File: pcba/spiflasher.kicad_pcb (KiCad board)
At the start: 2 copper layers, 62.5 x 25.7 mm, 41 parts, among them J1 USB_B_Micro, J2 Conn_02x04_Counter_Clockwise, J3 Conn_01x10, J4 Conn_01x10, U1 FT232H, U2 93LC56BT-I/OT, U3 TXB0104PW, Y1 12 MHz

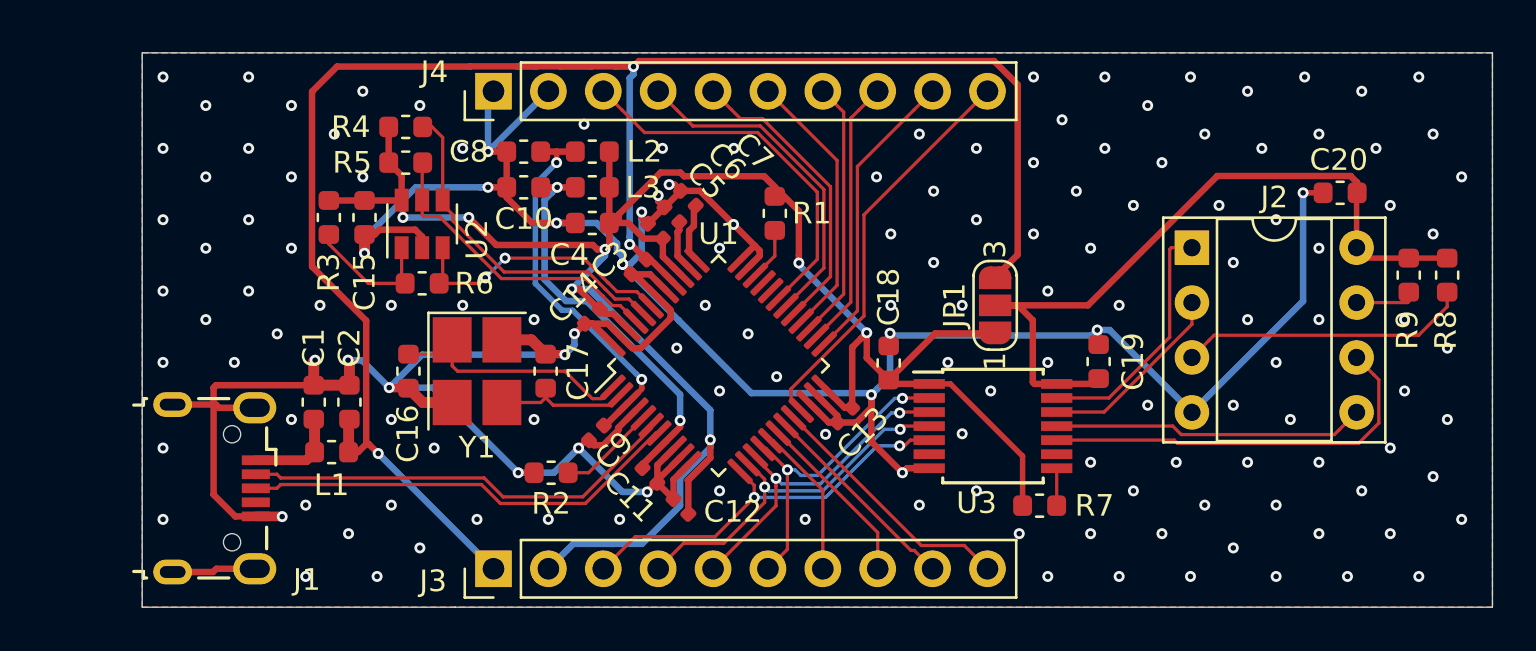
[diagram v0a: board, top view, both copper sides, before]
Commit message: Removed unnecessary components.
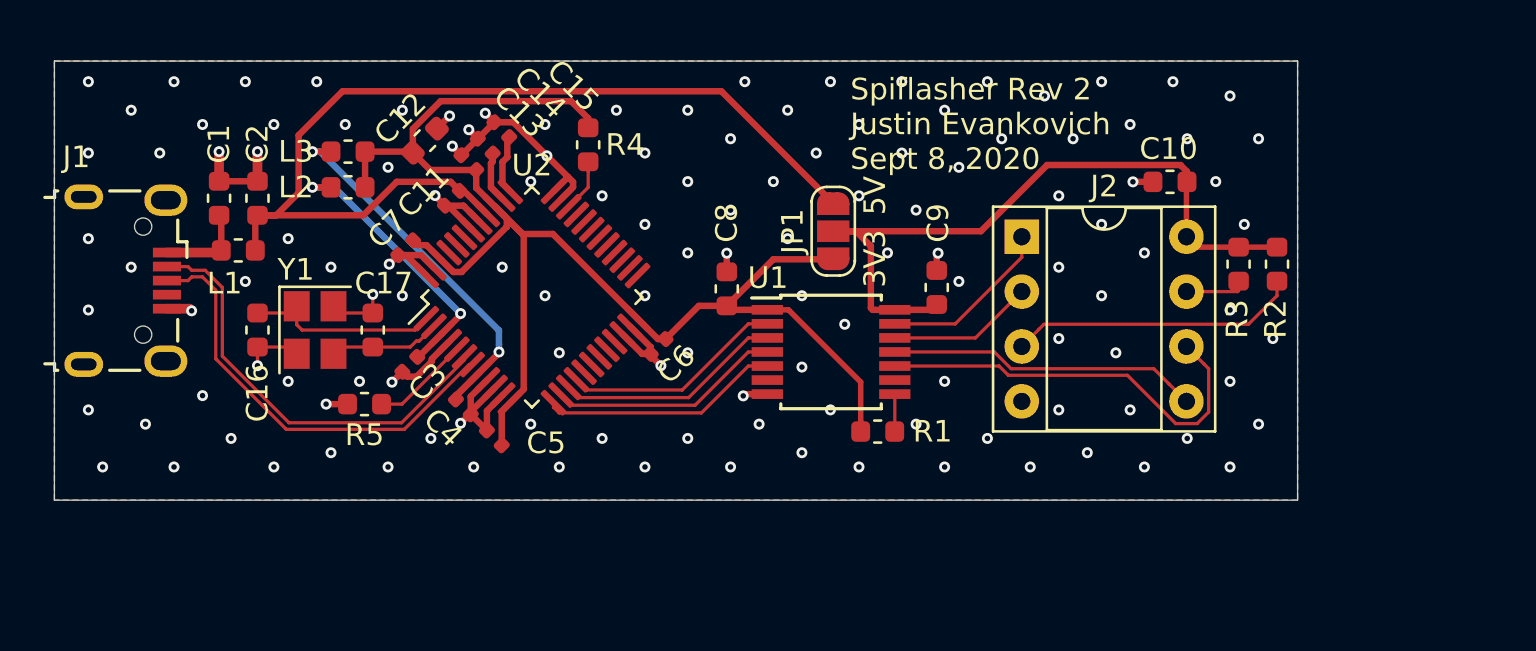
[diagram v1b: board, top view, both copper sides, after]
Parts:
- removed the C10 at (130.8, 97.3)
- removed the C15 at (123.4, 98.7)
- removed the C8 at (130.8, 95.6)
- removed J3, J4: Conn_01x10, Connector_PinHeader_2.54mm:PinHeader_1x10_P2.54mm_Vertical
- removed the R3 at (121.8, 98.7)
- removed the R4 at (125.3, 94.5)
- removed the R5 at (125.3, 96.1)
- removed R6: 2k, Resistor_SMD:R_0603_1608Metric
- removed the U2 at (126.1, 99.0)
- Y1: footprint Crystal:Crystal_SMD_3225-4Pin_3.2x2.5mm_HandSoldering -> Crystal:Crystal_SMD_3225-4Pin_3.2x2.5mm
- moved L2 11.4 mm to (122.7, 97.3)
- moved L3 11.4 mm to (122.7, 95.6)
- moved J1 10.5 mm to (112.4, 101.6)
- moved C1 10.4 mm to (116.7, 97.8)
- moved C2 10.4 mm to (118.5, 97.8)
- moved L1 10.3 mm to (117.6, 100.2)
- moved C6 9.20 mm to (137.0, 104.6)
- moved C7 9.20 mm to (125.3, 100.1)
- moved C11 9.20 mm to (127.5, 97.8)
- moved R5 9.20 mm to (123.4, 107.3)
- moved C14 9.20 mm to (129.0, 95.4)
- moved C15 9.20 mm to (129.8, 94.6)
- moved C4 9.20 mm to (128.0, 107.4)
- moved U2 9.20 mm to (131.2, 102.4)
- moved C13 9.20 mm to (128.3, 96.1)
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- renumbered C20 to C10, C3 to C11, C4 to C12, C5 to C13, C6 to C14, C7 to C15, C9 to C3, C11 to C4, C12 to C5, C13 to C6, C14 to C7, C18 to C8, C19 to C9, R7 to R1, R8 to R2, R9 to R3, R1 to R4, R2 to R5, U3 to U1, U1 to U2
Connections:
- U2 pad 17: Net-(J3-Pad7) -> (no net)
- U2 pad 18: Net-(J3-Pad8) -> (no net)
- U2 pad 19: Net-(J3-Pad9) -> (no net)
- U2 pad 20: Net-(J3-Pad10) -> (no net)
- U2 pad 21: Net-(J4-Pad10) -> (no net)
- U2 pad 25: Net-(J4-Pad9) -> (no net)
- U2 pad 26: Net-(J4-Pad8) -> (no net)
- U2 pad 27: Net-(J4-Pad7) -> (no net)
- U2 pad 28: Net-(J4-Pad6) -> (no net)
- U2 pad 29: Net-(J4-Pad5) -> (no net)
- U2 pad 30: Net-(J4-Pad4) -> (no net)
- U2 pad 31: Net-(J4-Pad3) -> (no net)
- U2 pad 43: Net-(R6-Pad2) -> (no net)
- U2 pad 44: Net-(R4-Pad2) (its old number) -> (no net)
- U2 pad 45: Net-(R5-Pad2) -> (no net)
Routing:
- net GND: track 186.0 -> 51.1 mm, vias 156 -> 130
- net VBUS: track 83.7 -> 47.2 mm, vias 3 -> 0
- net +3V3: track 100.1 -> 68.4 mm, vias 7 -> 0
- net Net-(J4-Pad10): track 18.7 -> 0.00 mm
- net Net-(J4-Pad3): track 17.5 -> 0.00 mm
- net Net-(R4-Pad2) (its old number): track 15.8 -> 0.00 mm
- net Net-(J4-Pad4): track 15.7 -> 0.00 mm
- net Net-(R5-Pad2): track 14.4 -> 0.00 mm
- net Net-(J4-Pad5): track 13.8 -> 0.00 mm
- net Net-(J4-Pad9): track 13.8 -> 0.00 mm
- net Net-(R6-Pad2): track 12.9 -> 0.00 mm, vias 2 -> 0
- net Net-(J4-Pad6): track 12.7 -> 0.00 mm
- net Net-(J4-Pad8): track 12.5 -> 0.00 mm
- net Net-(J4-Pad7): track 12.1 -> 0.00 mm
- net Net-(J3-Pad10): track 11.9 -> 0.00 mm
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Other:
- board size 62.5 x 25.7 mm -> 57.5 x 20.3 mm
- board text added: "Spiflasher Rev 2 Justin Evankovich Sept 8, 2020"
